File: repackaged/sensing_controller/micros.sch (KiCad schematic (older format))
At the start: 27 parts

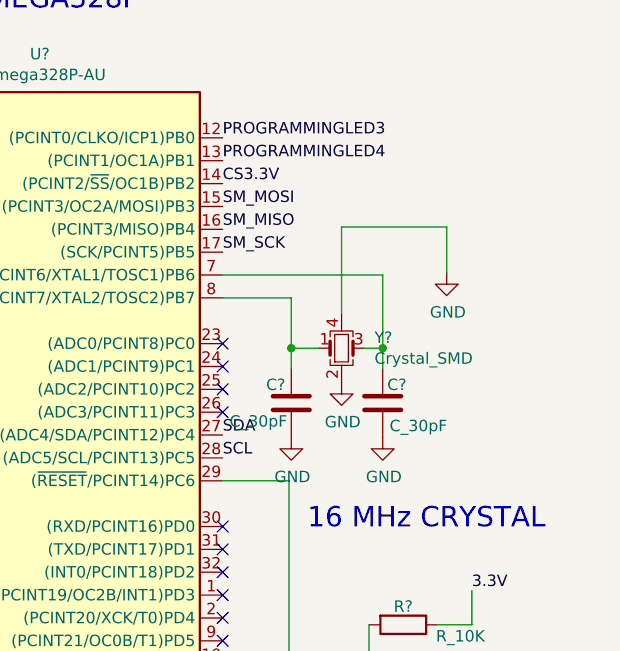
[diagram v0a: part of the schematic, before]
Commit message: Work on micros.sch
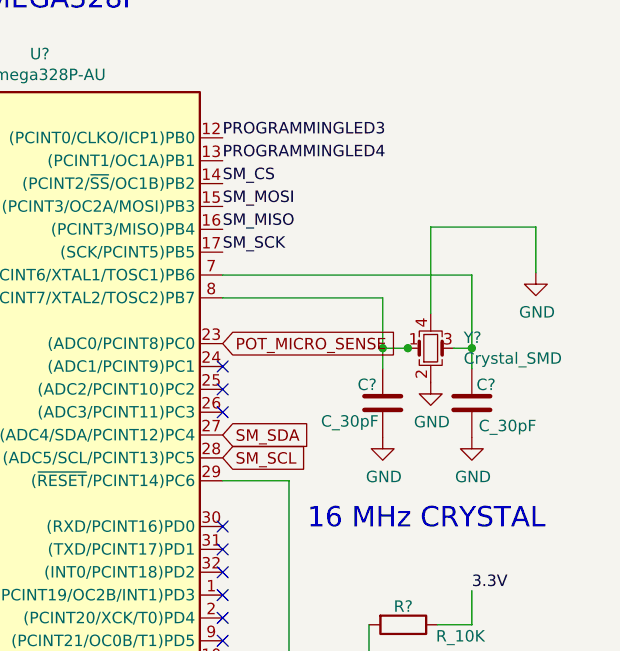
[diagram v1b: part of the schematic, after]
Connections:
- net CS3.3V: no longer U?.14 ((PCINT2/~SS~/OC1B)PB2)
- net POT_MICRO_SENSE: now reaches U?.23 ((ADC0/PCINT8)PC0)
- net SCL renamed SM_SCL
- net SDA renamed SM_SDA
- new net SM_CS: U?.14 ((PCINT2/~SS~/OC1B)PB2)
- no-connect marks 25 -> 24
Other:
- moved on the sheet: C?, Y?
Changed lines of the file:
@@
 $EndDescr
 Text Label 9610 1550 0    50   ~ 0
-CS3.3V
+SM_CS
 Text Label 7570 980  0    50   ~ 0
 3.3V
@@
 NoConn ~ 9610 2450
 NoConn ~ 9610 2350
-NoConn ~ 9610 2250
 Wire Wire Line
 	7570 1650 7570 2520
@@
 Text Label 9610 1850 0    50   ~ 0
 SM_SCK
-Text Label 9610 2750 0    50   ~ 0
-SCL
-Text Label 9610 2650 0    50   ~ 0
-SDA
 Wire Wire Line
 	9900 2850 9610 2850
@@
 L power:GND #PWR?
 U 1 1 60A51E4F
-P 10590 1940
-F 0 "#PWR?" H 10590 1690 50  0001 C CNN
-F 1 "GND" H 10595 1767 50  0000 C CNN
-F 2 "" H 10590 1940 50  0001 C CNN
-F 3 "" H 10590 1940 50  0001 C CNN
-	1    10590 1940
+P 10980 1940
+F 0 "#PWR?" H 10980 1690 50  0001 C CNN
+F 1 "GND" H 10985 1767 50  0000 C CNN
+F 2 "" H 10980 1940 50  0001 C CNN
+F 3 "" H 10980 1940 50  0001 C CNN
+	1    10980 1940
 	1    0    0    -1
 $EndComp
@@
 L power:GND #PWR?
 U 1 1 60A51E5E
+P 10700 2660
+F 0 "#PWR?" H 10700 2410 50  0001 C CNN
+F 1 "GND" H 10705 2487 50  0000 C CNN
+F 2 "" H 10700 2660 50  0001 C CNN
+F 3 "" H 10700 2660 50  0001 C CNN
+	1    10700 2660
+	1    0    0    -1
+$EndComp
+$Comp
+L power:GND #PWR?
+U 1 1 60A51E64
 P 10310 2660
 F 0 "#PWR?" H 10310 2410 50  0001 C CNN
@@
 $EndComp
 $Comp
-L power:GND #PWR?
-U 1 1 60A51E64
-P 9910 2660
-F 0 "#PWR?" H 9910 2410 50  0001 C CNN
-F 1 "GND" H 9915 2487 50  0000 C CNN
-F 2 "" H 9910 2660 50  0001 C CNN
-F 3 "" H 9910 2660 50  0001 C CNN
-	1    9910 2660
-	1    0    0    -1
-$EndComp
-$Comp
 L formula:C_30pF C?
 U 1 1 60A51E6D
-P 10310 2510
-F 0 "C?" H 10330 2590 50  0000 L CNN
-F 1 "C_30pF" H 10340 2410 50  0000 L CNN
-F 2 "footprints:C_0805_OEM" H 10348 2360 50  0001 C CNN
-F 3 "https://media.digikey.com/pdf/Data%20Sheets/Samsung%20PDFs/CL_Series_MLCC_ds.pdf" H 10335 2610 50  0001 C CNN
-F 4 "DK" H 10310 2510 60  0001 C CNN "MFN"
-F 5 "1276-1130-1-ND" H 10310 2510 60  0001 C CNN "MPN"
-F 6 "https://www.digikey.com/product-detail/en/samsung-electro-mechanics-america-inc/CL21C300JBANNNC/1276-1130-1-ND/3889216" H 10735 3010 60  0001 C CNN "PurchasingLink"
-	1    10310 2510
-	1    0    0    -1
-$EndComp
-$Comp
-L formula:C_30pF C?
-U 1 1 60A51E76
-P 9910 2510
-F 0 "C?" H 9800 2590 50  0000 L CNN
-F 1 "C_30pF" H 9640 2430 50  0000 L CNN
-F 2 "footprints:C_0805_OEM" H 9948 2360 50  0001 C CNN
-F 3 "https://media.digikey.com/pdf/Data%20Sheets/Samsung%20PDFs/CL_Series_MLCC_ds.pdf" H 9935 2610 50  0001 C CNN
-F 4 "DK" H 9910 2510 60  0001 C CNN "MFN"
-F 5 "1276-1130-1-ND" H 9910 2510 60  0001 C CNN "MPN"
-F 6 "https://www.digikey.com/product-detail/en/samsung-electro-mechanics-america-inc/CL21C300JBANNNC/1276-1130-1-ND/3889216" H 10335 3010 60  0001 C CNN "PurchasingLink"
-	1    9910 2510
-	1    0    0    -1
-$EndComp
-$Comp
-L formula:Crystal_SMD Y?
-U 1 1 60A51E7F
-P 10130 2270
-F 0 "Y?" H 10274 2316 50  0000 L CNN
-F 1 "Crystal_SMD" H 10274 2225 50  0000 L CNN
-F 2 "footprints:Crystal_SMD_FA238" H 10080 2345 50  0001 C CNN
-F 3 "http://www.txccorp.com/download/products/quartz_crystals/2015TXC_7M_17.pdf" H 10180 2445 50  0001 C CNN
-F 4 "DK" H 10130 2270 60  0001 C CNN "MFN"
-F 5 "887-1125-1-ND" H 10130 2270 60  0001 C CNN "MPN"
-F 6 "https://www.digikey.com/product-detail/en/txc-corporation/7M-16.000MAAJ-T/887-1125-1-ND/2119014" H 10580 2845 60  0001 C CNN "PurchasingLink"
-	1    10130 2270
-	1    0    0    -1
-$EndComp
-Wire Wire Line
-	9910 2050 9910 2270
-Wire Wire Line
-	10310 1950 10310 2270
-Wire Wire Line
-	10030 2270 9910 2270
-Connection ~ 9910 2270
-Wire Wire Line
-	9910 2270 9910 2360
-Wire Wire Line
-	10230 2270 10310 2270
-Connection ~ 10310 2270
-Wire Wire Line
-	10310 2270 10310 2360
-$Comp
-L power:GND #PWR?
-U 1 1 60A51E8D
-P 10130 2420
-F 0 "#PWR?" H 10130 2170 50  0001 C CNN
-F 1 "GND" H 10135 2247 50  0000 C CNN
-F 2 "" H 10130 2420 50  0001 C CNN
-F 3 "" H 10130 2420 50  0001 C CNN
-	1    10130 2420
-	1    0    0    -1
-$EndComp
-Wire Wire Line
-	9610 2050 9910 2050
-Wire Wire Line
-	10310 1950 9610 1950
-Wire Wire Line
-	10130 1740 10130 2120
-Wire Wire Line
-	10130 1740 10590 1740
-Wire Wire Line
-	10590 1740 10590 1940
+P 10700 2510
+F 0 "C?" H 10720 2590 50  0000 L CNN
+F 1 "C_30pF" H 10730 2410 50  0000 L CNN
+F 2 "footprints:C_0805_OEM" H 10738 2360 50  0001 C CNN
+F 3 "https://media.digikey.com/pdf/Data%20Sheets/Samsung%20PDFs/CL_Series_MLCC_ds.pdf" H 10725 2610 50  0001 C CNN
+F 4 "DK" H 10700 2510 60  0001 C CNN "MFN"
+F 5 "1276-1130-1-ND" H 10700 2510 60  0001 C CNN "MPN"
+F 6 "https://www.digikey.com/product-detail/en/samsung-electro-mechanics-america-inc/CL21C300JBANNNC/1276-1130-1-ND/3889216" H 11125 3010 60  0001 C CNN "PurchasingLink"
+	1    10700 2510
+	1    0    0    -1
+$EndComp
+Wire Wire Line
+	10700 1950 10700 2270
+Wire Wire Line
+	10620 2270 10700 2270
+Connection ~ 10700 2270
+Wire Wire Line
+	10700 2270 10700 2360
+Wire Wire Line
+	10520 1740 10980 1740
+Wire Wire Line
+	10980 1740 10980 1940
 Wire Wire Line
 	8010 3450 7740 3450
@@
 	1050 1100 1350 1100
 Connection ~ 1050 1400
+Text GLabel 9610 2250 2    50   Input ~ 0
+POT_MICRO_SENSE
+Wire Wire Line
+	10310 2050 10310 2270
+$Comp
+L formula:Crystal_SMD Y?
+U 1 1 60A51E7F
+P 10520 2270
+F 0 "Y?" H 10664 2316 50  0000 L CNN
+F 1 "Crystal_SMD" H 10664 2225 50  0000 L CNN
+F 2 "footprints:Crystal_SMD_FA238" H 10470 2345 50  0001 C CNN
+F 3 "http://www.txccorp.com/download/products/quartz_crystals/2015TXC_7M_17.pdf" H 10570 2445 50  0001 C CNN
+F 4 "DK" H 10520 2270 60  0001 C CNN "MFN"
+F 5 "887-1125-1-ND" H 10520 2270 60  0001 C CNN "MPN"
+F 6 "https://www.digikey.com/product-detail/en/txc-corporation/7M-16.000MAAJ-T/887-1125-1-ND/2119014" H 10970 2845 60  0001 C CNN "PurchasingLink"
+	1    10520 2270
+	1    0    0    -1
+$EndComp
+Wire Wire Line
+	10520 1740 10520 2120
+$Comp
+L power:GND #PWR?
+U 1 1 60A51E8D
+P 10520 2420
+F 0 "#PWR?" H 10520 2170 50  0001 C CNN
+F 1 "GND" H 10525 2247 50  0000 C CNN
+F 2 "" H 10520 2420 50  0001 C CNN
+F 3 "" H 10520 2420 50  0001 C CNN
+	1    10520 2420
+	1    0    0    -1
+$EndComp
+$Comp
+L formula:C_30pF C?
+U 1 1 60A51E76
+P 10310 2510
+F 0 "C?" H 10200 2590 50  0000 L CNN
+F 1 "C_30pF" H 10040 2430 50  0000 L CNN
+F 2 "footprints:C_0805_OEM" H 10348 2360 50  0001 C CNN
+F 3 "https://media.digikey.com/pdf/Data%20Sheets/Samsung%20PDFs/CL_Series_MLCC_ds.pdf" H 10335 2610 50  0001 C CNN
+F 4 "DK" H 10310 2510 60  0001 C CNN "MFN"
+F 5 "1276-1130-1-ND" H 10310 2510 60  0001 C CNN "MPN"
+F 6 "https://www.digikey.com/product-detail/en/samsung-electro-mechanics-america-inc/CL21C300JBANNNC/1276-1130-1-ND/3889216" H 10735 3010 60  0001 C CNN "PurchasingLink"
+	1    10310 2510
+	1    0    0    -1
+$EndComp
+Wire Wire Line
+	10430 2270 10420 2270
+Connection ~ 10310 2270
+Wire Wire Line
+	10310 2270 10310 2360
+Connection ~ 10420 2270
+Wire Wire Line
+	10420 2270 10310 2270
+Wire Wire Line
+	9610 1950 10700 1950
+Wire Wire Line
+	9610 2050 10310 2050
+Text GLabel 9610 2650 2    50   Input ~ 0
+SM_SDA
+Text GLabel 9610 2750 2    50   Input ~ 0
+SM_SCL
 $EndSCHEMATC
